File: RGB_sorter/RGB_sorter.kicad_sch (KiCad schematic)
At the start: 50 parts, among them J1 Servo, J10 TCS34725, J11 IR sensor, J2 Power, J3 Motor A, J4 Motor B, J6 LCD, J8 Conn_01x05_Pin, SW1 START, SW2 RESET, SW3 STOP, U1 L298N, U2 L7805, U3 ULN2003, U4 NUCLEO64-F411RE

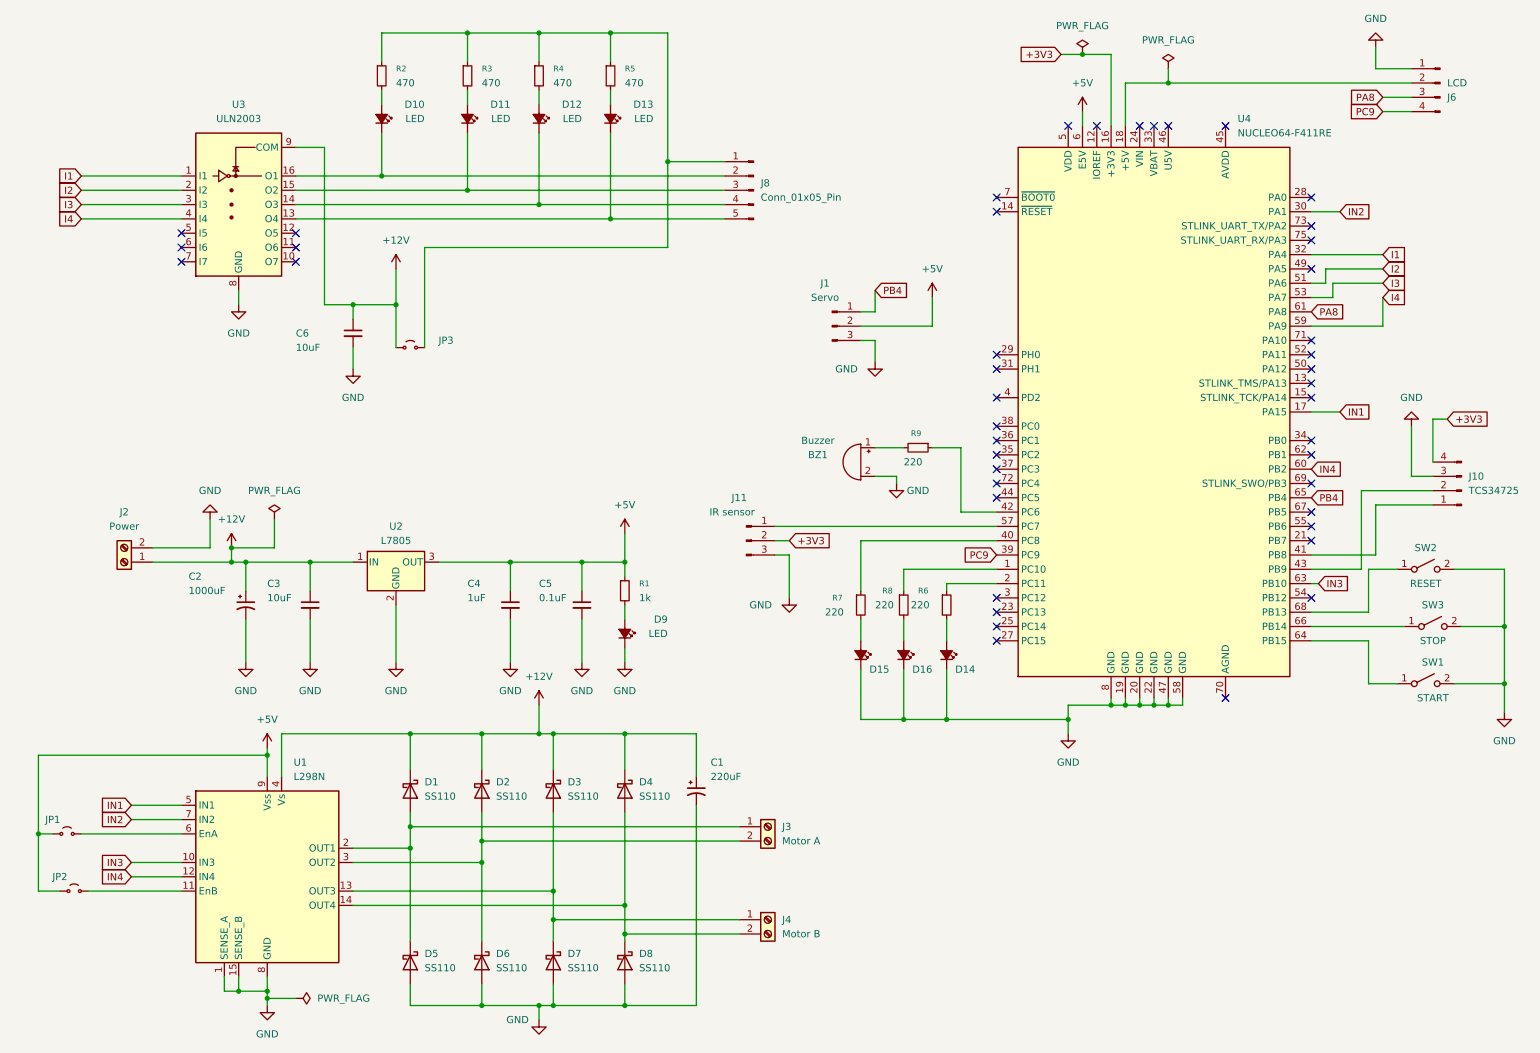
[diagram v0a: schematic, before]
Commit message: Upgrade PCB-a
Shematic i PCB edit
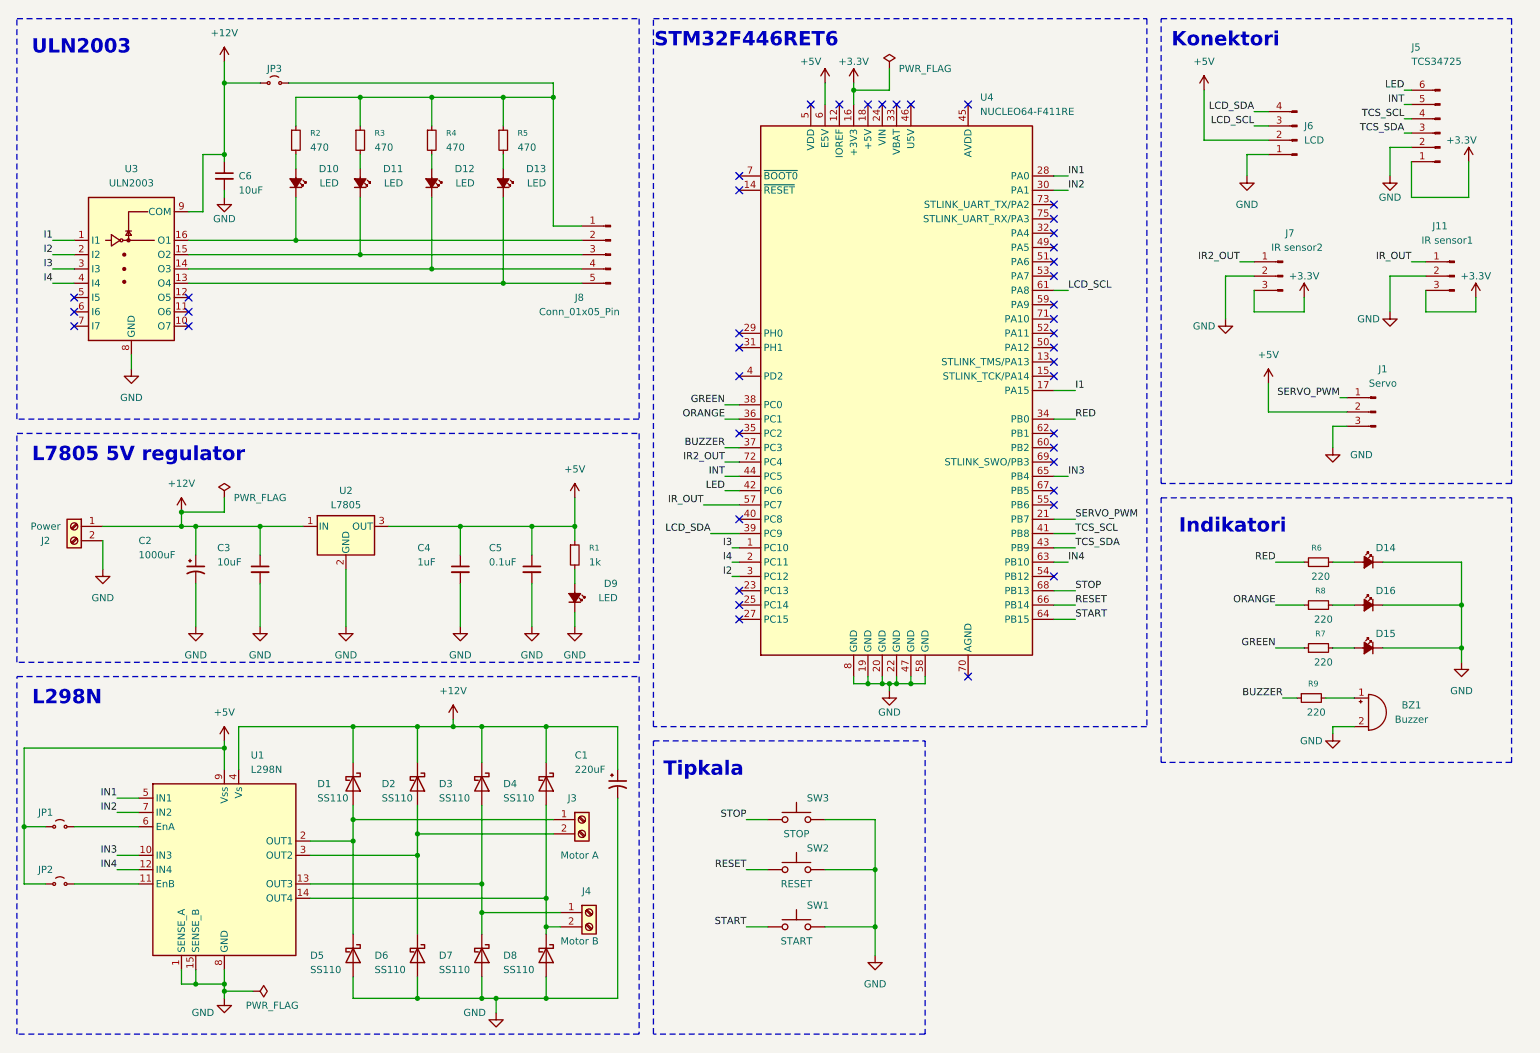
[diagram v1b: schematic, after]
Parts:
- removed J10: TCS34725, Connector_PinHeader_2.54mm:PinHeader_1x04_P2.54mm_Vertical, symbol Connector:Conn_01x04_Pin
- removed SW1: START, Button_Switch_THT:SW_PUSH-12mm_Wuerth-430476085716, symbol Switch:SW_SPST
- removed SW2: RESET, Button_Switch_THT:SW_PUSH-12mm_Wuerth-430476085716, symbol Switch:SW_SPST
- removed SW3: STOP, Button_Switch_THT:SW_PUSH-12mm_Wuerth-430476085716, symbol Switch:SW_SPST
- added J5: TCS34725, Connector_PinHeader_2.54mm:PinHeader_1x06_P2.54mm_Vertical, symbol Connector:Conn_01x06_Pin
- added J7: IR sensor2, Connector_PinHeader_2.54mm:PinHeader_1x03_P2.54mm_Vertical, symbol Connector:Conn_01x03_Pin
- added SW1: START, Button_Switch_THT:SW_PUSH-12mm_Wuerth-430476085716, symbol Switch:SW_Push
- added SW2: RESET, Button_Switch_THT:SW_PUSH-12mm_Wuerth-430476085716, symbol Switch:SW_Push
- added SW3: STOP, Button_Switch_THT:SW_PUSH-12mm_Wuerth-430476085716, symbol Switch:SW_Push
- D16: value LED_Blue -> LED_Orange
- J11: value IR sensor -> IR sensor1
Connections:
- net +5V: now also J6.2 (Pin_2)
- net GND: now also J11.2 (Pin_2), J5.2 (Pin_2), J7.2 (Pin_2), SW1.2, SW2.2, SW3.2; no longer J11.3 (Pin_3)
- net I1: now also U4.17 (PA15); no longer U4.32 (PA4)
- net I2: now also U4.3 (PC12); no longer U4.51 (PA6)
- net I3: now also U4.1 (PC10); no longer U4.53 (PA7)
- net I4: now also U4.2 (PC11); no longer U4.59 (PA9)
- net IN1: now also U4.28 (PA0); no longer U4.17 (PA15)
- net IN3: now also U4.65 (PB4); no longer U4.63 (PB10)
- net IN4: now also U4.63 (PB10); no longer U4.60 (PB2)
- net TCS_SCL: now reaches U4.41 (PB8)
- net TCS_SCL: now also J5.4 (Pin_4)
- net TCS_SDA: now reaches U4.43 (PB9)
- net TCS_SDA: now also J5.3 (Pin_3)
- net at U4.40 (PC8): no longer R7.1
- net ORANGE: now reaches R8.1
- net ORANGE: now also U4.36 (PC1); no longer U4.1 (PC10)
- net at U4.18 (+5V): no longer J6.2 (Pin_2)
- net RED: now reaches R6.1
- net RED: now also U4.34 (PB0); no longer U4.2 (PC11)
- net SERVO_PWM: now reaches U4.21 (PB7)
- net SERVO_PWM: now also J1.1 (Pin_1)
- net BUZZER: now reaches U4.37 (PC3)
- net BUZZER: now also R9.1
- net GREEN: now reaches U4.38 (PC0)
- net GREEN: now also R7.1
- net LED: now reaches U4.42 (PC6)
- net LED: now also J5.6 (Pin_6); no longer R9.1
- net INT: now reaches U4.44 (PC5)
- net INT: now also J5.5 (Pin_5)
- net IR_OUT: now reaches J11.1 (Pin_1), U4.57 (PC7)
- net START: now reaches U4.64 (PB15)
- net START: now also SW1.1
- net RESET: now reaches U4.66 (PB14)
- net RESET: now also SW2.1
- net STOP: now reaches U4.68 (PB13)
- net STOP: now also SW3.1
- net IR2_OUT: now reaches U4.72 (PC4)
- net IR2_OUT: now also J7.1 (Pin_1)
- net +3V3 renamed +3.3V
- net +3.3V: now also J11.3 (Pin_3), J5.1 (Pin_1), J7.3 (Pin_3); no longer J11.2 (Pin_2)
- net PA8 renamed LCD_SCL
- removed net PB4: J1.1 (Pin_1), U4.65 (PB4)
- net PC9 renamed LCD_SDA
- no-connect marks 44 -> 42
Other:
- note added: "Indikatori"
- note added: "Konektori"
- note added: "L298N"
- note added: "L7805 5V regulator"
- note added: "STM32F446RET6"
- note added: "Tipkala"
- note added: "ULN2003"
- moved on the sheet: BZ1, C1, C2, C3, C4, C5, C6, D1, D10, D11, D12, D13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
